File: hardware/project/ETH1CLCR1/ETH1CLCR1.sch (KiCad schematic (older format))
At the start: 0 parts

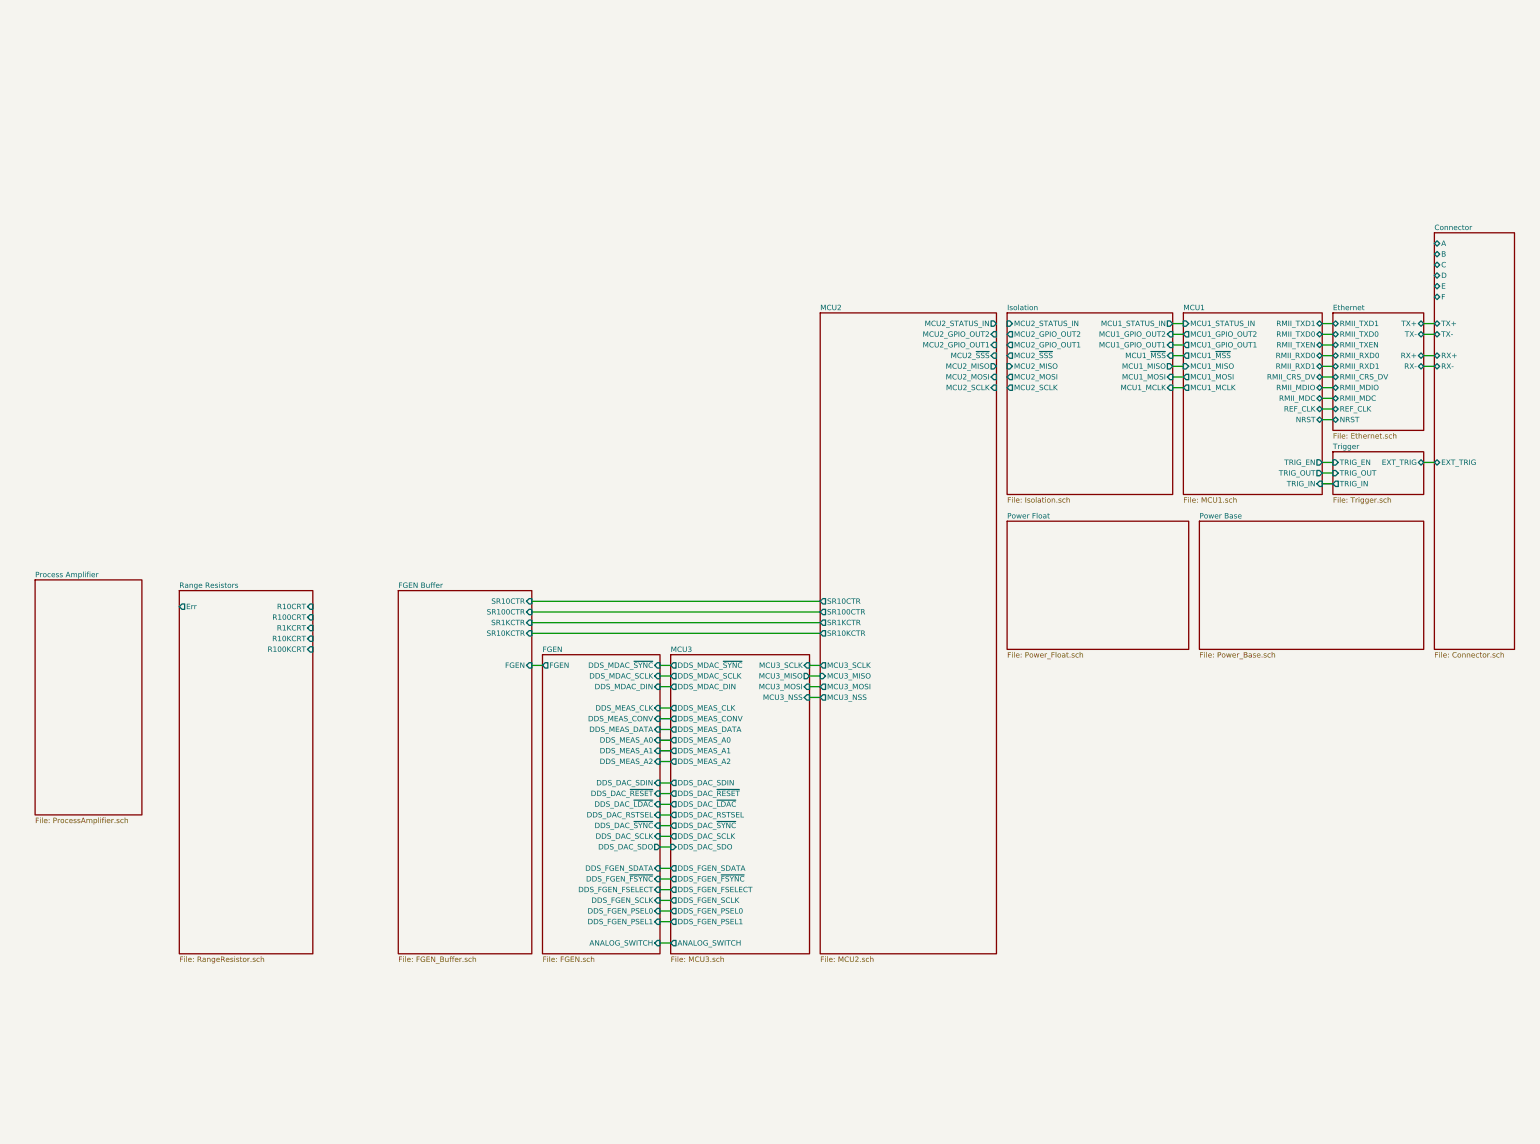
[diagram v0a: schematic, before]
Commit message: Schematic design
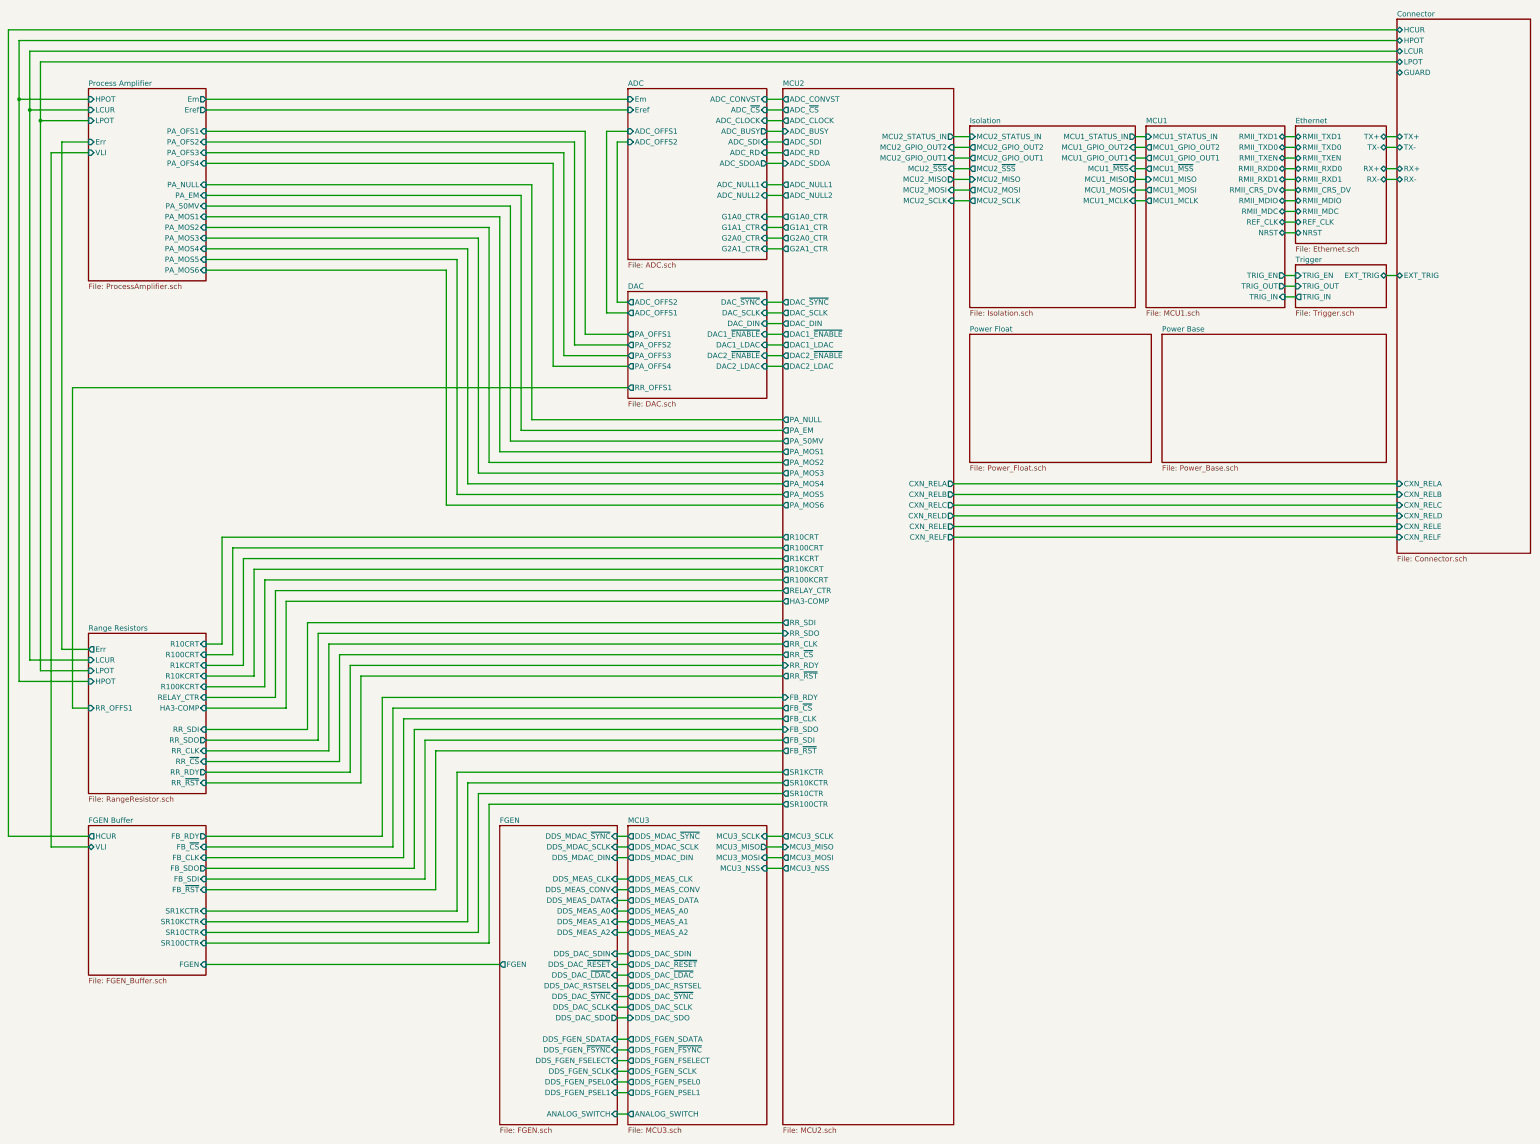
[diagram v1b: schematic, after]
